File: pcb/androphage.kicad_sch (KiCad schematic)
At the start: 0 parts

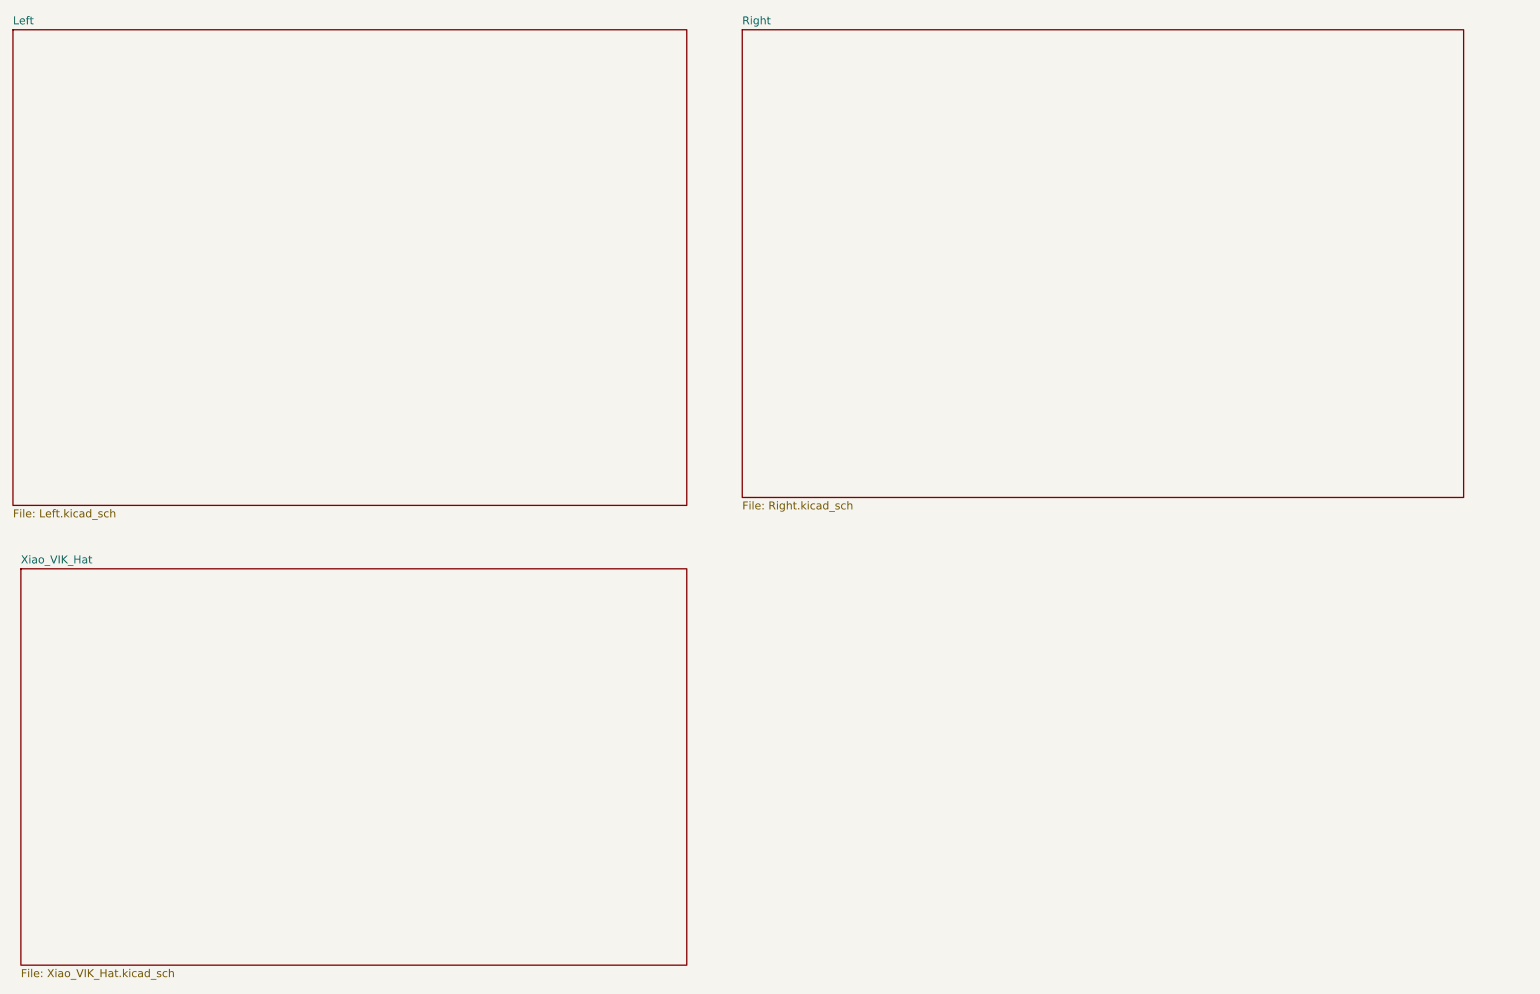
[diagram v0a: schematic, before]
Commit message: Tentatively finish PCB design.
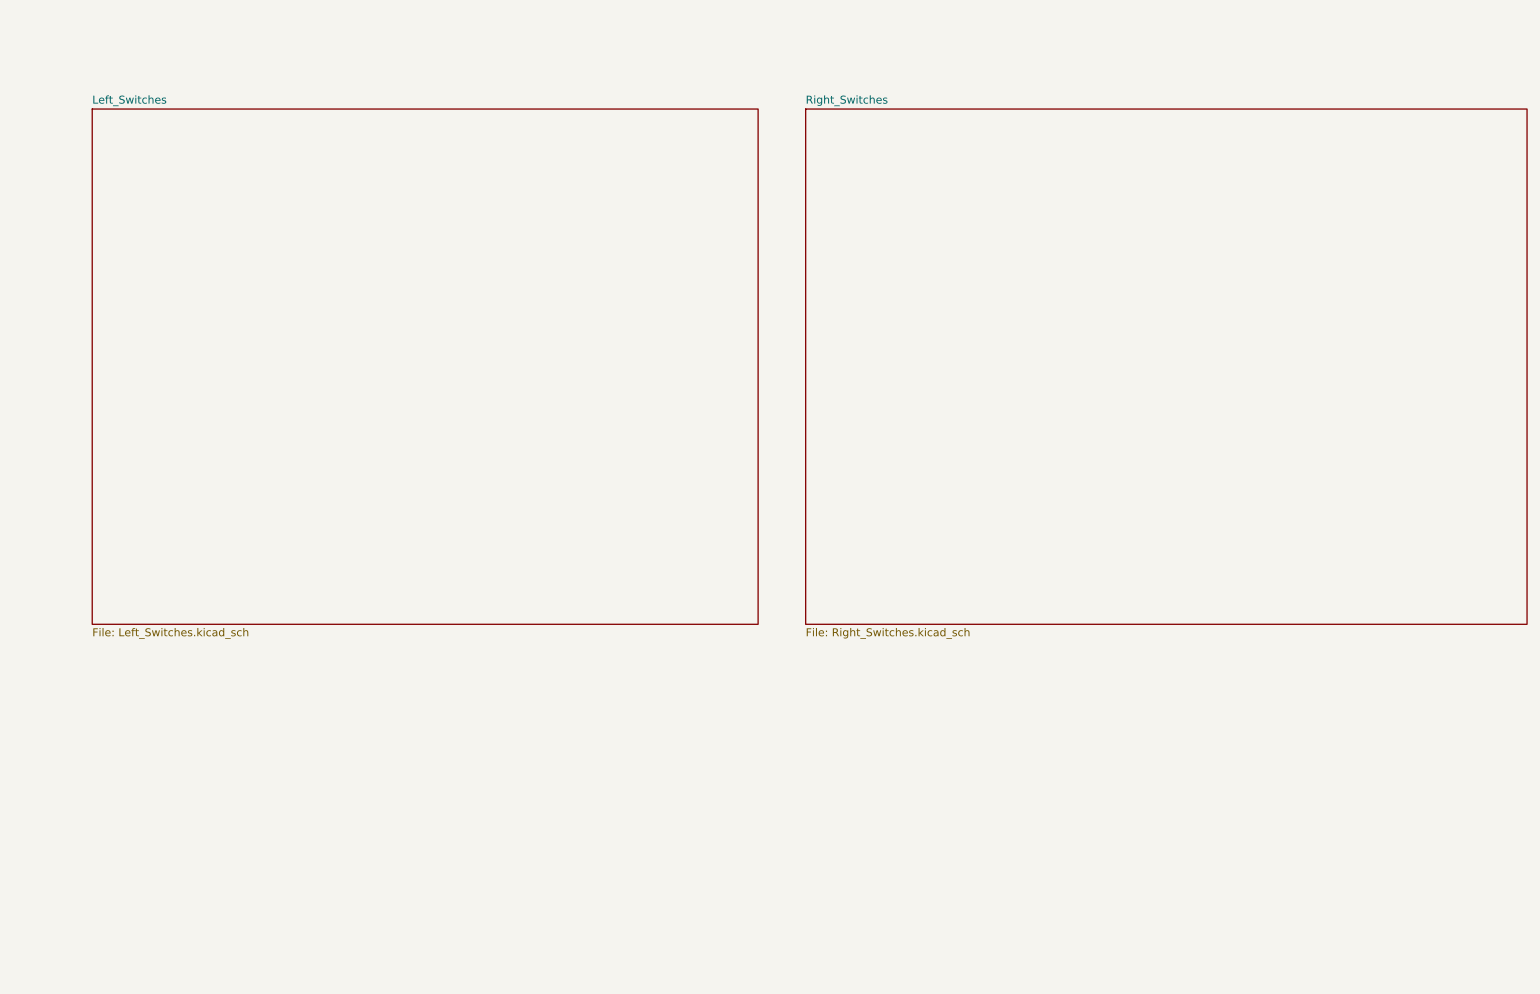
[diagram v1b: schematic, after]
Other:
- removed sheet Left
- removed sheet Right
- removed sheet Xiao_VIK_Hat
- added sheet Left_Switches (Left_Switches.kicad_sch)
- added sheet Right_Switches (Right_Switches.kicad_sch)
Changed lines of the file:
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@@
 	(paper "A4")
 	(sheet
-		(at 3.81 3.81)
-		(size 107.95 76.2)
+		(at 130.81 16.51)
+		(size 115.57 82.55)
 		(exclude_from_sim no)
 		(in_bom yes)
@@
 			(color 0 0 0 0.0000)
 		)
-		(property "Sheetname" "Left"
-			(at 3.81 3.0984 0)
+		(property "Sheetname" "Right_Switches"
+			(at 130.81 15.7984 0)
 			(effects
 				(font
@@
 			)
 		)
-		(property "Sheetfile" "Left.kicad_sch"
-			(at 3.81 80.5946 0)
+		(property "Sheetfile" "Right_Switches.kicad_sch"
+			(at 130.81 99.6446 0)
 			(effects
 				(font
@@
 			(project "androphage"
 				(path "/75763295-000b-439c-b3ba-6692a992e76d"
-					(page "2")
+					(page "5")
 				)
 			)
@@
 	)
 	(sheet
-		(at 120.65 3.81)
-		(size 115.57 74.93)
+		(at 16.51 16.51)
+		(size 106.68 82.55)
 		(exclude_from_sim no)
 		(in_bom yes)
@@
 			(color 0 0 0 0.0000)
 		)
-		(property "Sheetname" "Right"
-			(at 120.65 3.0984 0)
+		(property "Sheetname" "Left_Switches"
+			(at 16.51 15.7984 0)
 			(effects
 				(font
@@
 			)
 		)
-		(property "Sheetfile" "Right.kicad_sch"
-			(at 120.65 79.3246 0)
+		(property "Sheetfile" "Left_Switches.kicad_sch"
+			(at 16.51 99.6446 0)
 			(effects
 				(font
@@
 			)
 		)
-		(property "Field2" ""
-			(at 120.65 3.81 0)
-			(effects
-				(font
-					(size 1.27 1.27)
-				)
-			)
-		)
-		(instances
-			(project "androphage"
-				(path "/75763295-000b-439c-b3ba-6692a992e76d"
-					(page "3")
-				)
-			)
-		)
-	)
-	(sheet
-		(at 5.08 90.17)
-		(size 106.68 63.5)
-		(exclude_from_sim no)
-		(in_bom yes)
-		(on_board yes)
-		(dnp no)
-		(fields_autoplaced yes)
-		(stroke
-			(width 0.1524)
-			(type solid)
-		)
-		(fill
-			(color 0 0 0 0.0000)
-		)
-		(property "Sheetname" "Xiao_VIK_Hat"
-			(at 5.08 89.4584 0)
-			(effects
-				(font
-					(size 1.27 1.27)
-				)
-				(justify left bottom)
-			)
-		)
-		(property "Sheetfile" "Xiao_VIK_Hat.kicad_sch"
-			(at 5.08 154.2546 0)
-			(effects
-				(font
-					(size 1.27 1.27)
-				)
-				(justify left top)
-			)
-		)
-		(property "Field2" ""
-			(at 5.08 90.17 0)
-			(effects
-				(font
-					(size 1.27 1.27)
-				)
-			)
-		)
